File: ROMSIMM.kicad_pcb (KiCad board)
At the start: 4 copper layers, 88.9 x 19 mm, 8 parts, among them J1 Conn_01x30, U1 511400, U2 511400

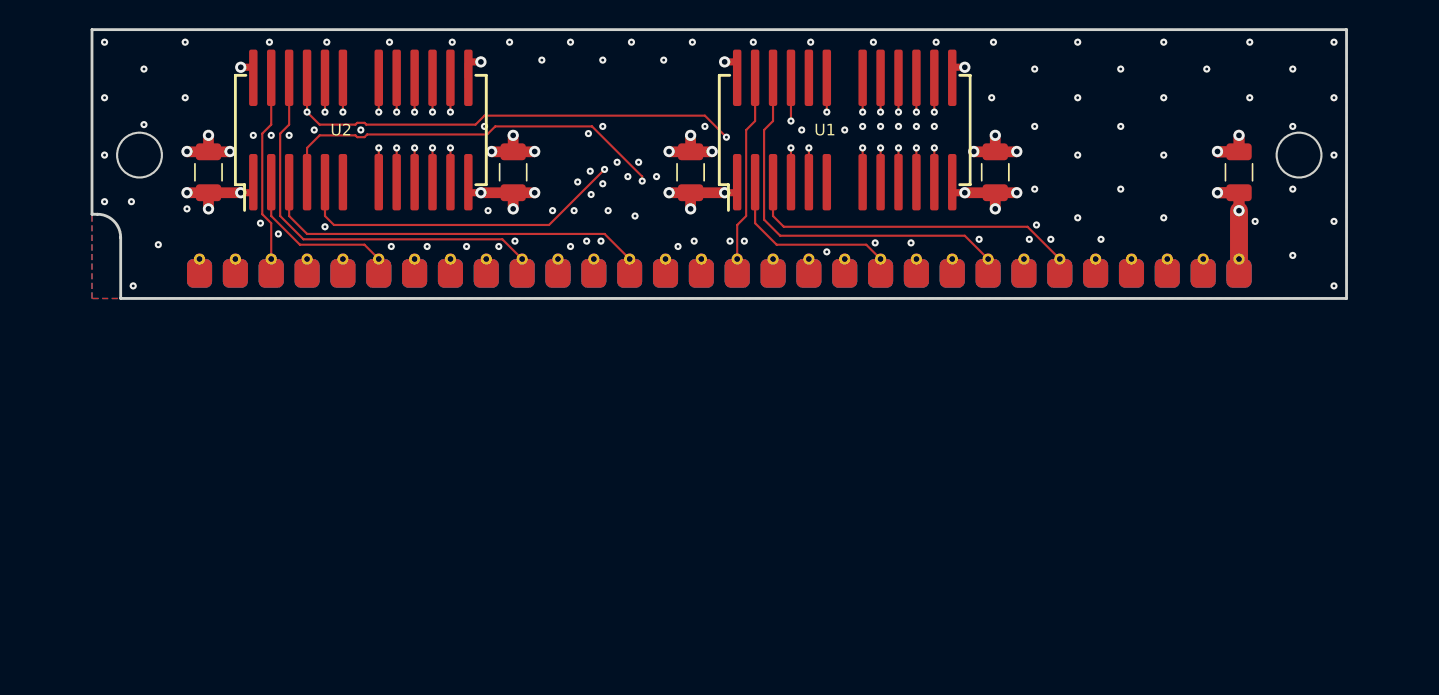
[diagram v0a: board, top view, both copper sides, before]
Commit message: asdsda
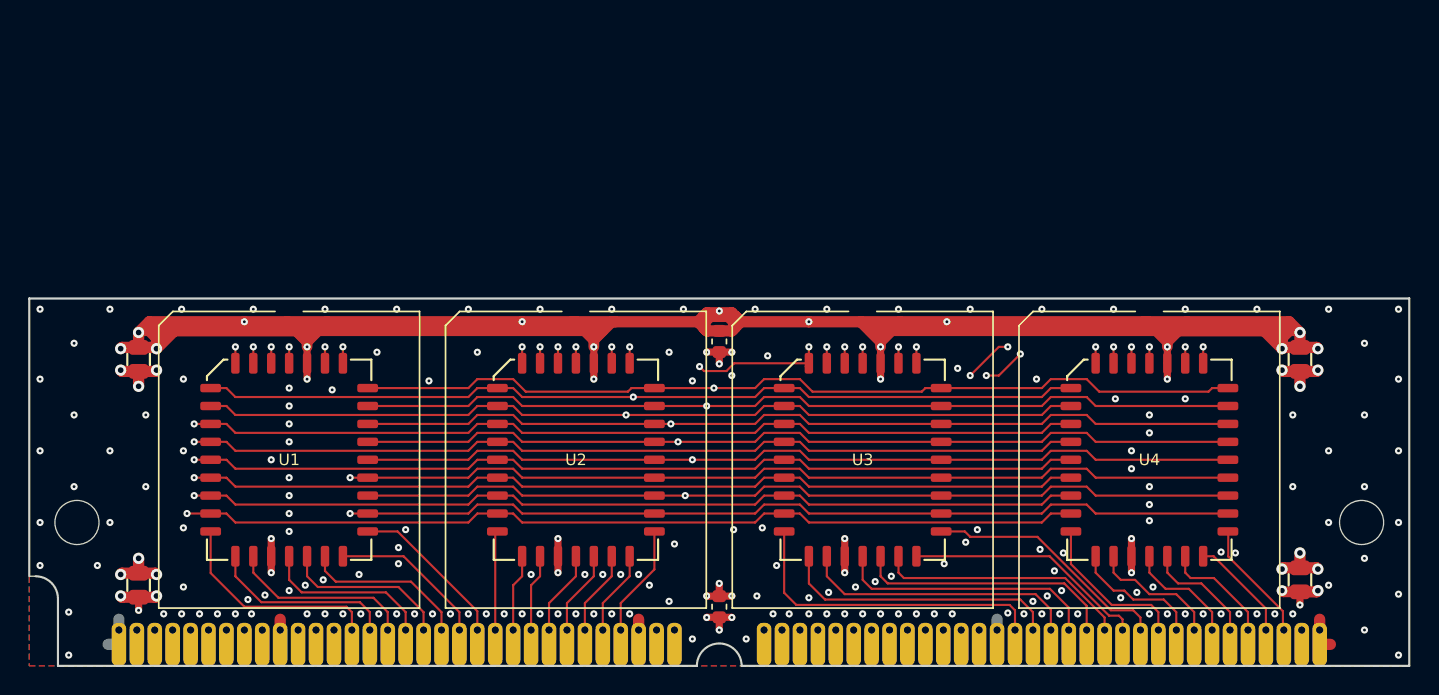
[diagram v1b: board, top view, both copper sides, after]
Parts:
- removed the C3 at (118.6, 92.7)
- removed the C3 at (140.2, 92.7)
- added C3: 10u, stdpads:C_0805, F.Cu at (161.8, 105.9)
- added C5: 2u2, stdpads:C_0603, F.Cu at (120.7, 123.4)
- added C6: 2u2, stdpads:C_0603, F.Cu at (120.7, 104.6)
- added H1: MountingHole, Conn:MH_125, F.Cu at (75.1, 117.5)
- added H2: MountingHole, Conn:MH_125, F.Cu at (166.2, 117.5)
- added U3: D15-8, stdpads:PLCC-32_SMDSocket, F.Cu at (130.8, 113.0)
- added U4: D7-0, stdpads:PLCC-32_SMDSocket, F.Cu at (151.1, 113.0)
- C1, C2, C4: value 100n -> 10u; footprint stdpads:C_1206 -> stdpads:C_0805
- J1: value Conn_01x30 -> ROM; footprint stdpads:SIMM-30_Edge -> stdpads:MacIIROMSIMM_Edge
- U1: value 511400 -> D31-24; footprint stdpads:SOJ-24-26-300mil -> stdpads:PLCC-32_SMDSocket
- U2: value 511400 -> D23-16; footprint stdpads:SOJ-24-26-300mil -> stdpads:PLCC-32_SMDSocket
- moved U1 45.8 mm to (90.2, 113.0), turned to 0 degrees
- moved C2 39.5 mm to (79.5, 121.9)
- moved C4 29.2 mm to (161.8, 121.5)
- moved U2 27.9 mm to (110.5, 113.0), turned to 0 degrees
- moved J1 27.8 mm to (120.7, 127.6)
- moved C1 14.2 mm to (79.5, 105.9), turned to 270 degrees
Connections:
- J1 pad 10: /D2 -> GND
- J1 pad 11: /1A6 -> /~CS~
- J1 pad 12: /1A1 -> /~OE~
- J1 pad 13: /D3 -> /~WE~
- J1 pad 14: /1A7 -> /D0
- J1 pad 15: /1A0 -> /D1
- J1 pad 16: /D4 -> /D2
- J1 pad 17: /1A8 -> /D3
- J1 pad 18: /1A10 -> /D4
- J1 pad 19: /1A9 -> /D5
- J1 pad 2: /~CAS~ -> /A0
- J1 pad 20: /D5 -> /D6
- J1 pad 21: /~WE~ -> /D7
- J1 pad 22: GND -> /D8
- J1 pad 23: /D6 -> /D9
- J1 pad 24: /A11 -> /D10
- J1 pad 25: /D7 -> /D11
- J1 pad 26: /QP -> /D12
- J1 pad 27: /~RAS~ -> /D13
- J1 pad 28: /~CASP~ -> /D14
- J1 pad 29: /DP -> /D15
- J1 pad 3: /D0 -> /A1
- J1 pad 30: +5V -> GND
- J1 pad 4: /1A4 -> /A2
- J1 pad 5: /1A3 -> /A3
- J1 pad 6: /D1 -> /A4
- J1 pad 7: /1A5 -> /A5
- J1 pad 8: /1A2 -> /A6
- J1 pad 9: GND -> /A7
- U1 pad 1: +5V -> /A20
- U1 pad 10: /1A1 -> /A4
- U1 pad 11: /1A2 -> /A3
- U1 pad 12: /1A3 -> /A2
- U1 pad 13: +5V -> /D0
- U1 pad 14: GND -> /D1
- U1 pad 15: /1A4 -> /D2
- U1 pad 16: /1A5 -> GND
- U1 pad 17: /1A6 -> /D3
- U1 pad 18: /1A7 -> /D4
- U1 pad 19: /1A8 -> /D5
- U1 pad 2: /D5 -> /A18
- U1 pad 21: /1A9 -> /D7
- U1 pad 22: GND -> /~CS~
- U1 pad 23: /~CAS~ -> /A12
- U1 pad 24: /D6 -> /~OE~
- U1 pad 25: /D4 -> /A13
- U1 pad 26: GND -> /A11
- U1 pad 3: /D7 -> /A17
- U1 pad 4: /~WE~ -> /A14
- U1 pad 5: /~RAS~ -> /A9
- U1 pad 6: Net-(U1-Pad6) -> /A8
- U1 pad 8: /1A10 -> /A6
- U1 pad 9: /1A0 -> /A5
- U2 pad 1: +5V -> /A20
- U2 pad 10: /1A1 -> /A4
- U2 pad 11: /1A0 -> /A3
- U2 pad 12: /1A10 -> /A2
- U2 pad 13: +5V -> /D8
- U2 pad 14: GND -> /D9
- U2 pad 15: /1A9 -> /D10
- U2 pad 16: /1A8 -> GND
- U2 pad 17: /1A7 -> /D11
- U2 pad 18: /1A6 -> /D12
- U2 pad 19: /1A5 -> /D13
- U2 pad 2: /D1 -> /A18
- U2 pad 21: /1A4 -> /D15
- U2 pad 22: GND -> /~CS~
- U2 pad 23: /~CAS~ -> /A12
- U2 pad 24: /D2 -> /~OE~
- U2 pad 25: /D0 -> /A13
- U2 pad 26: GND -> /A11
- U2 pad 3: /D3 -> /A17
- U2 pad 4: /~WE~ -> /A14
- U2 pad 5: /~RAS~ -> /A9
- U2 pad 6: Net-(U2-Pad6) -> /A8
- U2 pad 8: /1A3 -> /A6
- U2 pad 9: /1A2 -> /A5
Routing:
- net +5V: track 29.6 -> 234.6 mm, vias 14 -> 28
- net /A20: track 0.00 -> 106.3 mm, vias 0 -> 4
- net /A14: track 0.00 -> 101.8 mm, vias 0 -> 5
- net /A19: track 0.00 -> 100.8 mm, vias 0 -> 4
- net /A17: track 0.00 -> 94.9 mm, vias 0 -> 6
- net /A18: track 0.00 -> 94.4 mm, vias 0 -> 6
- net /A16: track 0.00 -> 85.2 mm, vias 0 -> 1
- net /A15: track 0.00 -> 82.7 mm, vias 0 -> 1
- net /A7: track 0.00 -> 80.3 mm, vias 0 -> 1
- net /A9: track 0.00 -> 80.3 mm, vias 0 -> 1
- net /A10: track 0.00 -> 79.9 mm, vias 0 -> 1
- net /A11: track 0.00 -> 78.9 mm, vias 0 -> 1
- net /A13: track 0.00 -> 78.8 mm, vias 0 -> 1
- net /A8: track 0.00 -> 78.7 mm, vias 0 -> 1
- net /A6: track 0.00 -> 78.5 mm, vias 0 -> 1
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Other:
- board size 88.9 x 19 mm -> 97.8 x 26 mm
- board text added: "4401A"
- board text added: "GW"
- board text added: "Garrett’s Workshop"
- board text added: "ROM SIMM"
- board text added: "for Mac II and SE/30"
